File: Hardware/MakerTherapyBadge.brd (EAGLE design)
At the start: 63.5 x 85.7 mm, 69 parts, among them J1 AVR_SPI_PROG_3X2NS, U1 ATMEGA328P_TQFP, U3 MCP73831.SOT23-5

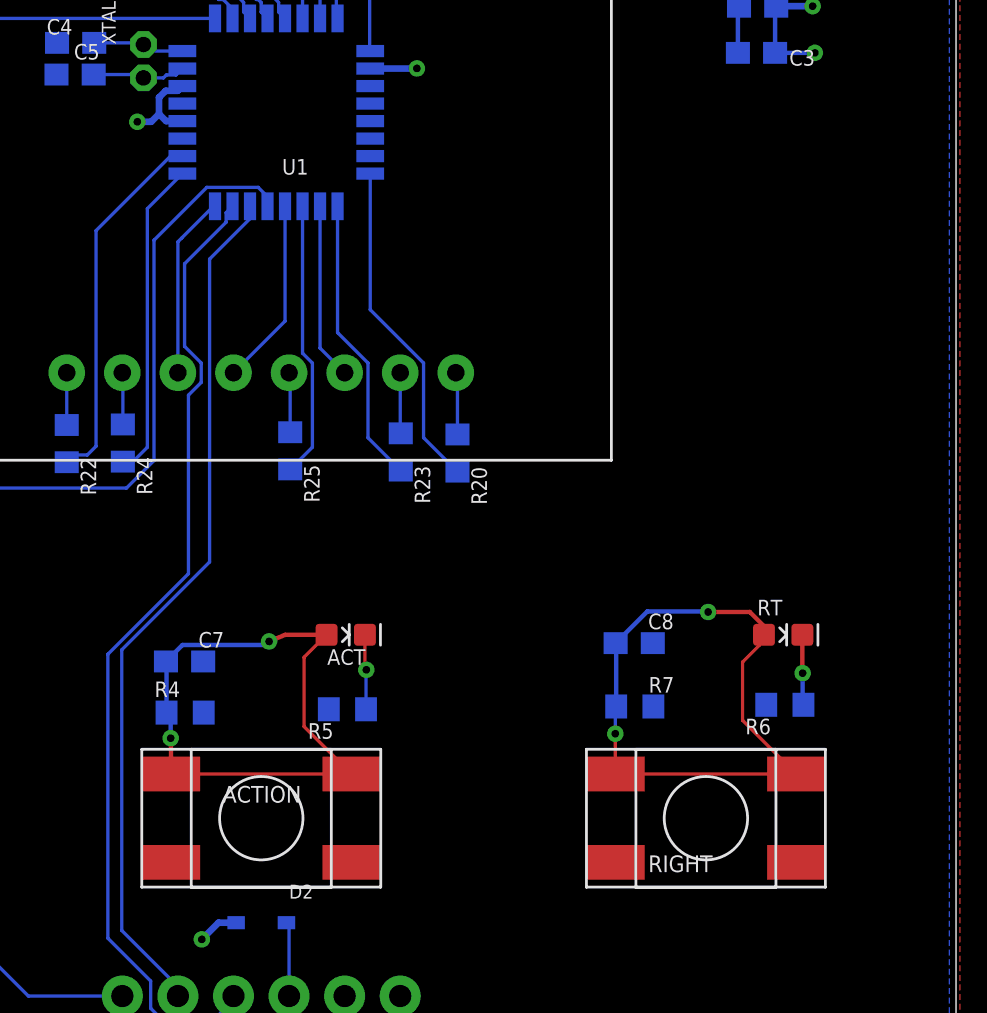
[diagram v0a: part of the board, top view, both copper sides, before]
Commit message: changes 4/17
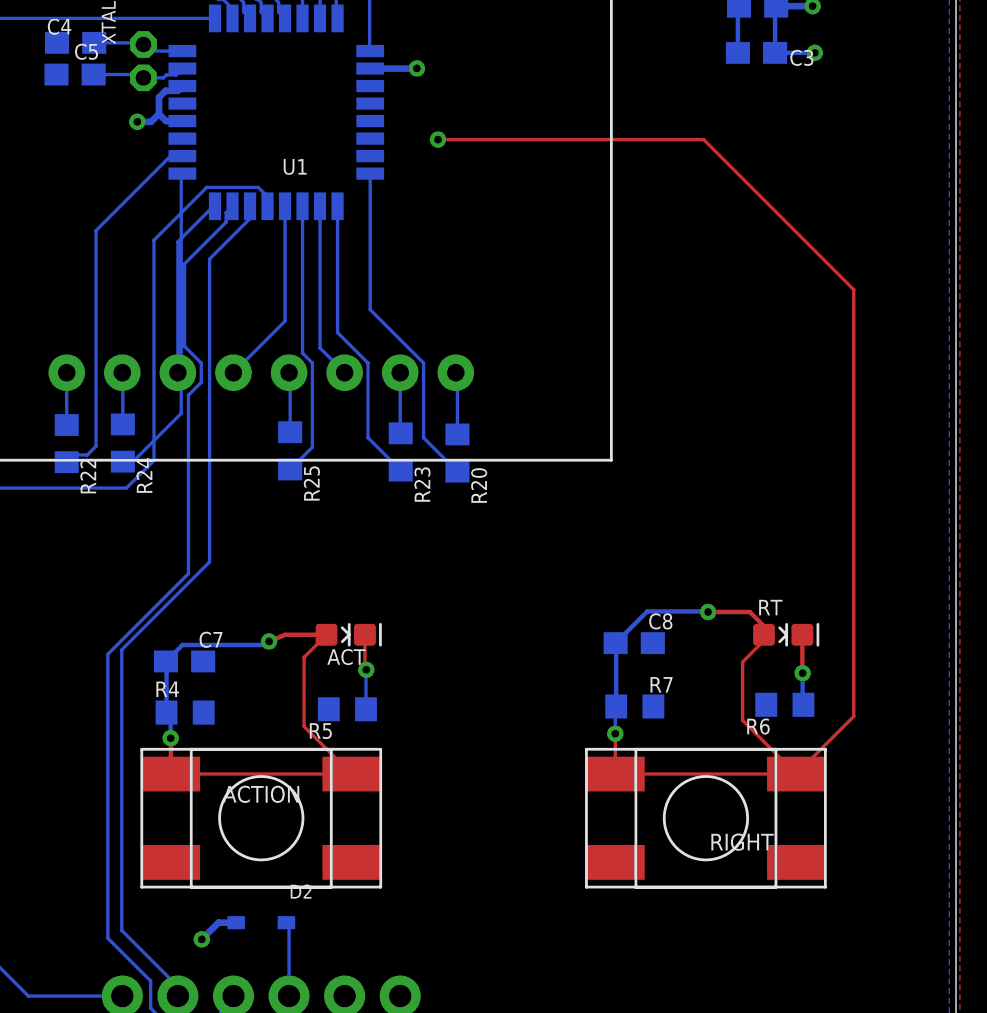
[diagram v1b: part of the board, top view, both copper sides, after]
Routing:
- net N$19: track 30.1 -> 75.1 mm, vias 2 -> 3
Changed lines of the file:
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@@
 </element>
 <element name="RIGHT" library="LinnesLab-Switches" package="SPST.KT11P4SM34LFS" value="" x="52.07" y="10.414" smashed="yes" rot="R180">
-<attribute name="NAME" x="52.3748" y="8.7122" size="0.762" layer="25" rot="R180"/>
+<attribute name="NAME" x="55.1688" y="9.7028" size="0.762" layer="25" rot="R180"/>
 <attribute name="VALUE" x="57.15" y="14.859" size="0.762" layer="27" rot="R180"/>
 </element>
 <element name="ACTION" library="LinnesLab-Switches" package="SPST.KT11P4SM34LFS" value="" x="31.75" y="10.414" smashed="yes" rot="R180">
+<attribute name="ACTION" value="" x="31.75" y="10.414" size="1.778" layer="27" rot="R180" display="off"/>
 <attribute name="NAME" x="33.5788" y="11.8872" size="0.762" layer="25" rot="R180"/>
 <attribute name="VALUE" x="36.83" y="14.859" size="0.762" layer="27" rot="R180"/>
@@
 <wire x1="47.9298" y1="14.2748" x2="47.9298" y2="15.4804" width="0.1524" layer="16"/>
 <wire x1="47.9298" y1="15.4804" x2="47.9688" y2="15.5194" width="0.1524" layer="16"/>
+<wire x1="56.1975" y1="12.434" x2="58.8264" y2="15.0629" width="0.1524" layer="1"/>
+<wire x1="58.8264" y1="15.0629" x2="58.8264" y2="34.5694" width="0.1524" layer="1"/>
+<wire x1="58.8264" y1="34.5694" x2="51.9684" y2="41.4274" width="0.1524" layer="1"/>
+<wire x1="51.9684" y1="41.4274" x2="39.8272" y2="41.4274" width="0.1524" layer="1"/>
+<via x="39.8272" y="41.4274" extent="1-16" drill="0.35"/>
 </signal>
 <signal name="N$20">
@@
 <contactref element="R24" pad="1"/>
 <contactref element="U1" pad="1"/>
-<wire x1="26.543" y1="38.2718" x2="28.1432" y2="39.872" width="0.1524" layer="16"/>
-<wire x1="26.543" y1="27.3659125" x2="26.543" y2="38.2718" width="0.1524" layer="16"/>
+<wire x1="28.0924" y1="39.8212" x2="28.1432" y2="39.872" width="0.1524" layer="16"/>
+<wire x1="28.0924" y1="28.9153125" x2="28.0924" y2="39.8212" width="0.1524" layer="16"/>
 <wire x1="25.4254" y1="26.709" x2="25.8860875" y2="26.709" width="0.1524" layer="16"/>
-<wire x1="25.8860875" y1="26.709" x2="26.543" y2="27.3659125" width="0.1524" layer="16"/>
+<wire x1="25.8860875" y1="26.709" x2="28.0924" y2="28.9153125" width="0.1524" layer="16"/>
 </signal>
 <signal name="LD7">
